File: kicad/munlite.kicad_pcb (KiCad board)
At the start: 2 copper layers, 53.8 x 29 mm, 21 parts, among them J1 Conn_Pover, J2 Conn_Pir, J3 Conn_Prog, J4 Conn_Opto, J5 Conn_Led, SW1 SW_Push, T1 IRLR2905TRPBF, U1 STM32L031F6Px, U2 AP2112K-3.3

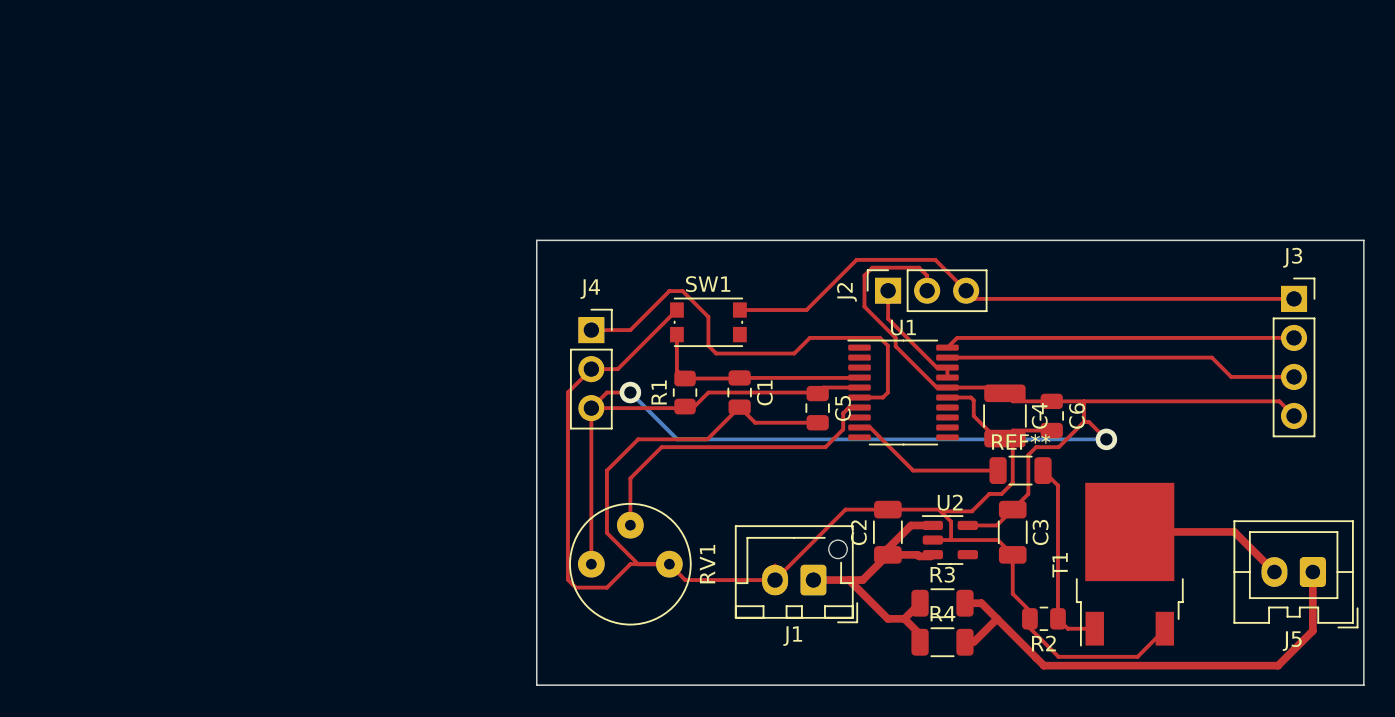
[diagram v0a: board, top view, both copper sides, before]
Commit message: update
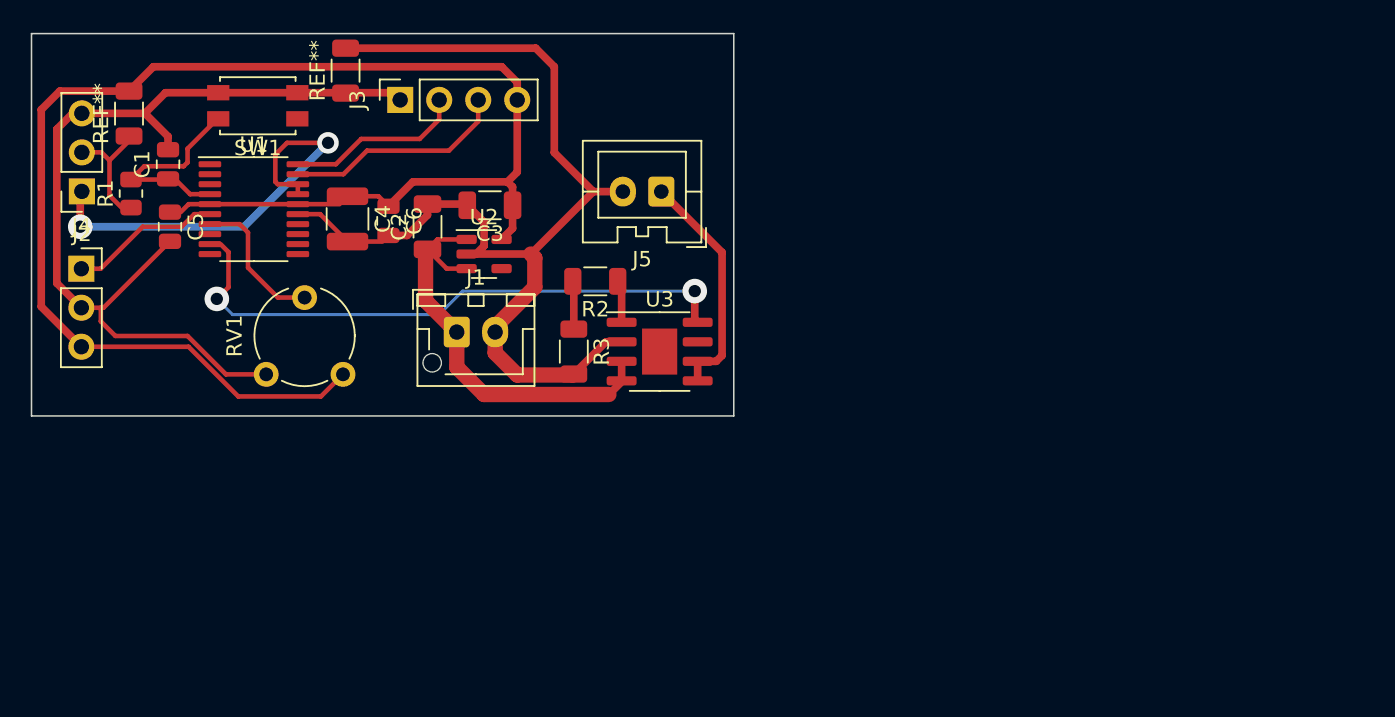
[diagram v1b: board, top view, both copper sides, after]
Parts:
- removed R4: 100, Resistor_SMD:R_1206_3216Metric
- removed the REF** at (104.1, 61.5)
- removed T1: IRLR2905TRPBF, Package_TO_SOT_SMD:TO-252-2
- added REF**: R_1206_3216Metric, Resistor_SMD:R_1206_3216Metric, F.Cu at (60.2, 35.4)
- added REF**: R_1206_3216Metric, Resistor_SMD:R_1206_3216Metric, F.Cu at (46.1, 38.2)
- added U3: CN5711, Package_SO:SOIC-8-1EP_3.9x4.9mm_P1.27mm_EP2.29x3mm, F.Cu at (80.6, 53.7)
- R2: value R -> 4.7 kOm; footprint Resistor_SMD:R_0805_2012Metric -> Resistor_SMD:R_1206_3216Metric
- R3: value 100 -> 2.2 kOm
- RV1: footprint Potentiometer_THT:Potentiometer_Bourns_3339P_Vertical_HandSoldering -> Potentiometer_THT:Potentiometer_Piher_PT-6-V_Vertical
- SW1: footprint Button_Switch_SMD:SW_Push_1P1T_NO_CK_KMR2 -> Button_Switch_SMD:SW_SPST_EVQP2
- moved J3 59.6 mm to (63.8, 37.3), turned to 90 degrees
- moved J2 52.9 mm to (43.0, 43.3), turned to 180 degrees
- moved J5 49.1 mm to (80.8, 43.3)
- moved C6 45.0 mm to (63.0, 45.2)
- moved C4 44.7 mm to (60.3, 45.1)
- moved U1 43.9 mm to (54.2, 44.5)
- moved C5 43.8 mm to (48.8, 45.6)
- moved C3 40.1 mm to (69.6, 44.2), turned to 180 degrees
- moved C1 40.1 mm to (48.6, 41.5), turned to 90 degrees
- moved R1 38.3 mm to (46.2, 43.4)
- moved R2 36.6 mm to (76.5, 49.1)
- moved C2 36.0 mm to (65.5, 45.6)
- moved U2 35.6 mm to (69.2, 47.4)
- moved J4 33.4 mm to (43.0, 48.3)
- moved SW1 32.5 mm to (54.5, 37.7), turned to 180 degrees
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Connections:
- C1 pad 1: Reset -> GND
- J5 pad 2: Net-(T1-Pad2) -> GND
- R1 pad 2: Reset -> GND
- R2 pad 1: Led -> Net-(R2-Pad1)
- R2 pad 2: GND -> Net-(R2-Pad2)
- R3 pad 1: +4V -> Net-(R2-Pad2)
- R3 pad 2: Net-(J5-Pad1) -> GND
- SW1 pad 2: Reset -> GND
- U1 pad 4: Reset -> GND
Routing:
- net Pir: track 7.66 -> 28.4 mm, vias 0 -> 2
- net Opto: track 28.8 -> 9.84 mm
- net Net-(J5-Pad1): track 31.8 -> 15.3 mm
- net Led: track 22.9 -> 39.1 mm, vias 0 -> 2
- net Reset: track 14.5 -> 0.00 mm
- net SWCLK: track 22.8 -> 11.7 mm
- net Sens: track 20.5 -> 9.48 mm
- net Net-(T1-Pad2): track 10.5 -> 0.00 mm
- net GND: track 153.3 -> 143.0 mm
- net SWDIO: track 23.1 -> 14.6 mm
- net +3V3: track 117.3 -> 110.9 mm, vias 2 -> 0
- net +4V: track 23.7 -> 27.6 mm
- net Net-(R2-Pad2): track 0.00 -> 3.14 mm
- net Net-(R2-Pad1): track 0.00 -> 2.77 mm
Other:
- board size 53.8 x 29 mm -> 45.7 x 24.9 mm
